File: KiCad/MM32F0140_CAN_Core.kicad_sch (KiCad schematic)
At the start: 0 parts

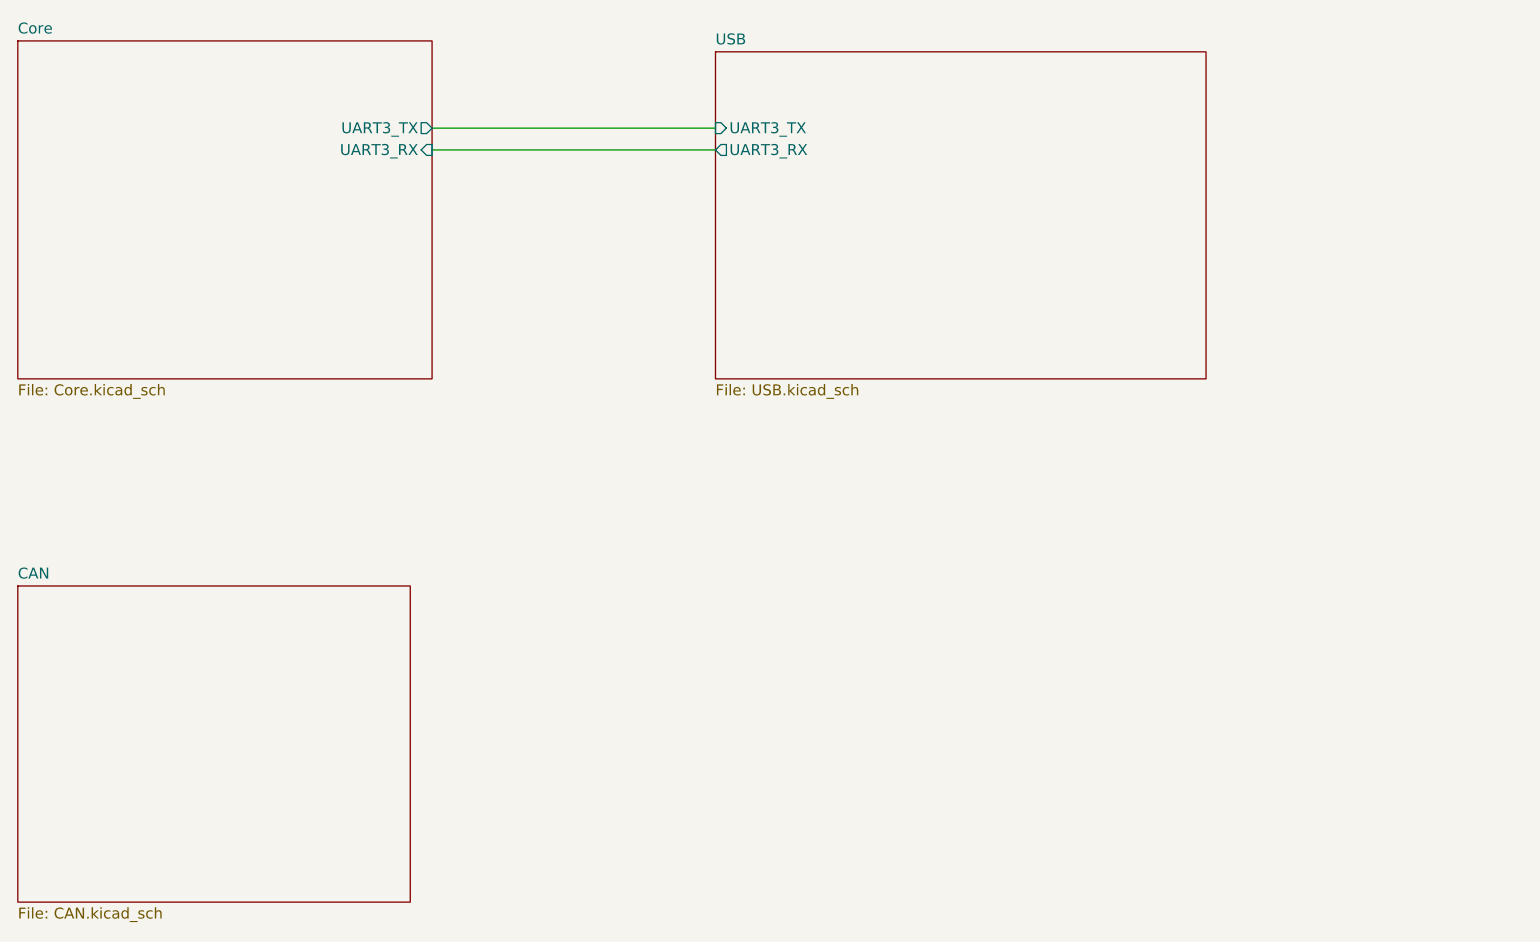
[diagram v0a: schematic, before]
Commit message: 原理图完成
2023.4.8:8:30
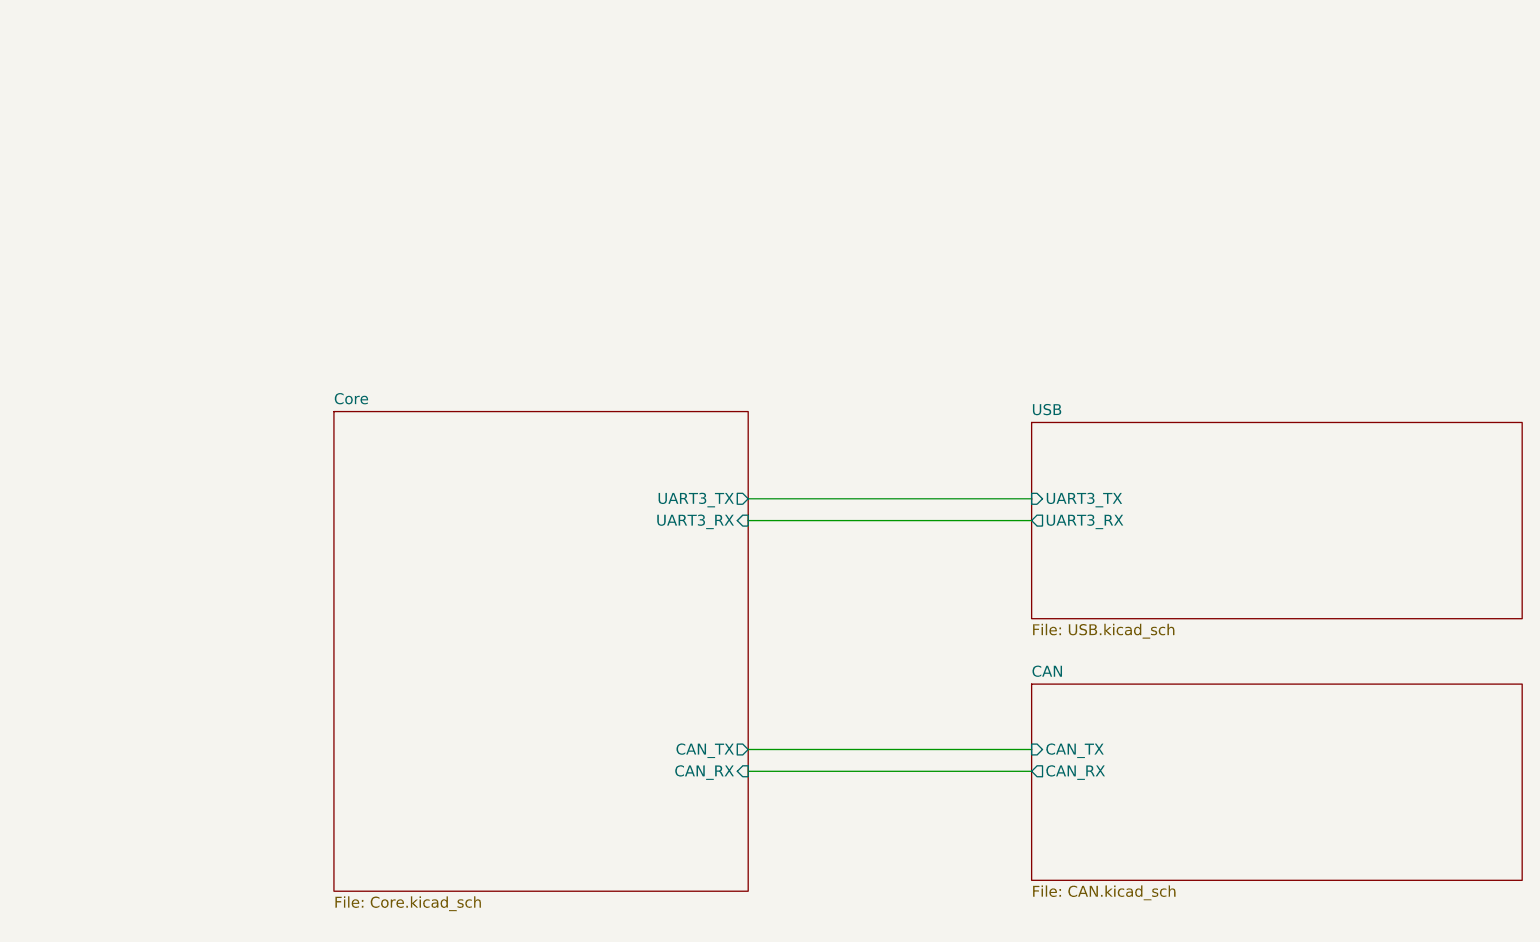
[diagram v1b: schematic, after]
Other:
- sheet CAN ports: added CAN_RX, CAN_TX; removed none
- sheet Core ports: added CAN_RX, CAN_TX; removed none
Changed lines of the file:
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@@
 (kicad_sch (version 20230121) (generator eeschema)
   (paper "A4")
-  (wire (pts (xy 80.01 34.29) (xy 113.03 34.29))
+  (wire (pts (xy 116.84 104.14) (xy 149.86 104.14))
     (stroke (width 0) (type default))
   )
-  (wire (pts (xy 80.01 31.75) (xy 113.03 31.75))
+  (wire (pts (xy 116.84 77.47) (xy 149.86 77.47))
     (stroke (width 0) (type default))
   )
-  (sheet (at 31.75 85.09) (size 45.72 36.83) (fields_autoplaced)
+  (wire (pts (xy 116.84 74.93) (xy 149.86 74.93))
+    (stroke (width 0) (type default))
+  )
+  (wire (pts (xy 116.84 106.68) (xy 149.86 106.68))
+    (stroke (width 0) (type default))
+  )
+  (sheet (at 149.86 96.52) (size 57.15 22.86) (fields_autoplaced)
     (stroke (width 0.1524) (type solid))
     (fill (color 0 0 0 0.0000))
-    (property "Sheetname" "CAN" (at 31.75 84.3784 0)
+    (property "Sheetname" "CAN" (at 149.86 95.8084 0)
       (effects (font (size 1.27 1.27)) (justify left bottom))
     )
-    (property "Sheetfile" "CAN.kicad_sch" (at 31.75 122.5046 0)
+    (property "Sheetfile" "CAN.kicad_sch" (at 149.86 119.9646 0)
       (effects (font (size 1.27 1.27)) (justify left top))
+    )
+    (pin "CAN_TX" input (at 149.86 104.14 180)
+      (effects (font (size 1.27 1.27)) (justify left))
+    )
+    (pin "CAN_RX" output (at 149.86 106.68 180)
+      (effects (font (size 1.27 1.27)) (justify left))
     )
     (instances
@@
     )
   )
-  (sheet (at 113.03 22.86) (size 57.15 38.1) (fields_autoplaced)
+  (sheet (at 149.86 66.04) (size 57.15 22.86) (fields_autoplaced)
     (stroke (width 0.1524) (type solid))
     (fill (color 0 0 0 0.0000))
-    (property "Sheetname" "USB" (at 113.03 22.1484 0)
+    (property "Sheetname" "USB" (at 149.86 65.3284 0)
       (effects (font (size 1.27 1.27)) (justify left bottom))
     )
-    (property "Sheetfile" "USB.kicad_sch" (at 113.03 61.5446 0)
+    (property "Sheetfile" "USB.kicad_sch" (at 149.86 89.4846 0)
       (effects (font (size 1.27 1.27)) (justify left top))
     )
-    (pin "UART3_RX" output (at 113.03 34.29 180)
+    (pin "UART3_RX" output (at 149.86 77.47 180)
       (effects (font (size 1.27 1.27)) (justify left))
     )
-    (pin "UART3_TX" input (at 113.03 31.75 180)
+    (pin "UART3_TX" input (at 149.86 74.93 180)
       (effects (font (size 1.27 1.27)) (justify left))
     )
@@
     )
   )
-  (sheet (at 31.75 21.59) (size 48.26 39.37) (fields_autoplaced)
+  (sheet (at 68.58 64.77) (size 48.26 55.88) (fields_autoplaced)
     (stroke (width 0.1524) (type solid))
     (fill (color 0 0 0 0.0000))
-    (property "Sheetname" "Core" (at 31.75 20.8784 0)
+    (property "Sheetname" "Core" (at 68.58 64.0584 0)
       (effects (font (size 1.27 1.27)) (justify left bottom))
     )
-    (property "Sheetfile" "Core.kicad_sch" (at 31.75 61.5446 0)
+    (property "Sheetfile" "Core.kicad_sch" (at 68.58 121.2346 0)
       (effects (font (size 1.27 1.27)) (justify left top))
     )
-    (pin "UART3_RX" input (at 80.01 34.29 0)
+    (pin "UART3_RX" input (at 116.84 77.47 0)
       (effects (font (size 1.27 1.27)) (justify right))
     )
-    (pin "UART3_TX" output (at 80.01 31.75 0)
+    (pin "UART3_TX" output (at 116.84 74.93 0)
       (effects (font (size 1.27 1.27)) (justify right))
     )
+    (pin "CAN_TX" output (at 116.84 104.14 0)
+      (effects (font (size 1.27 1.27)) (justify right))
+    )
+    (pin "CAN_RX" input (at 116.84 106.68 0)
+      (effects (font (size 1.27 1.27)) (justify right))
+    )
